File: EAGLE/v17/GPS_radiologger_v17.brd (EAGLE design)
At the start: 40.4 x 26.1 mm, 44 parts, among them IC4 CAT24M01HU5I-GT3, U1 TYPEABZ, U2 BMA400, U4 SPV1050, U5 BME680BME680, U6 CAM-M8Q-0

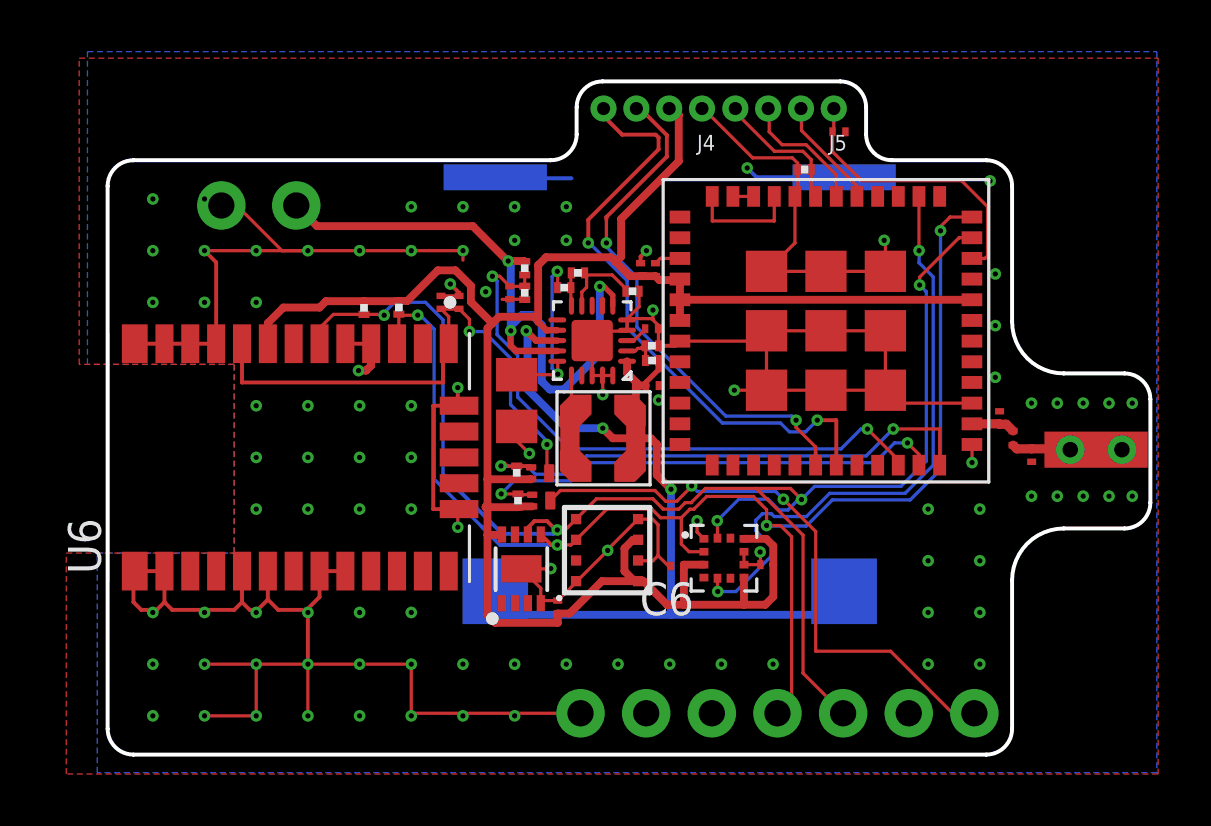
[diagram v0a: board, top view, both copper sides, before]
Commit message: recent board updates
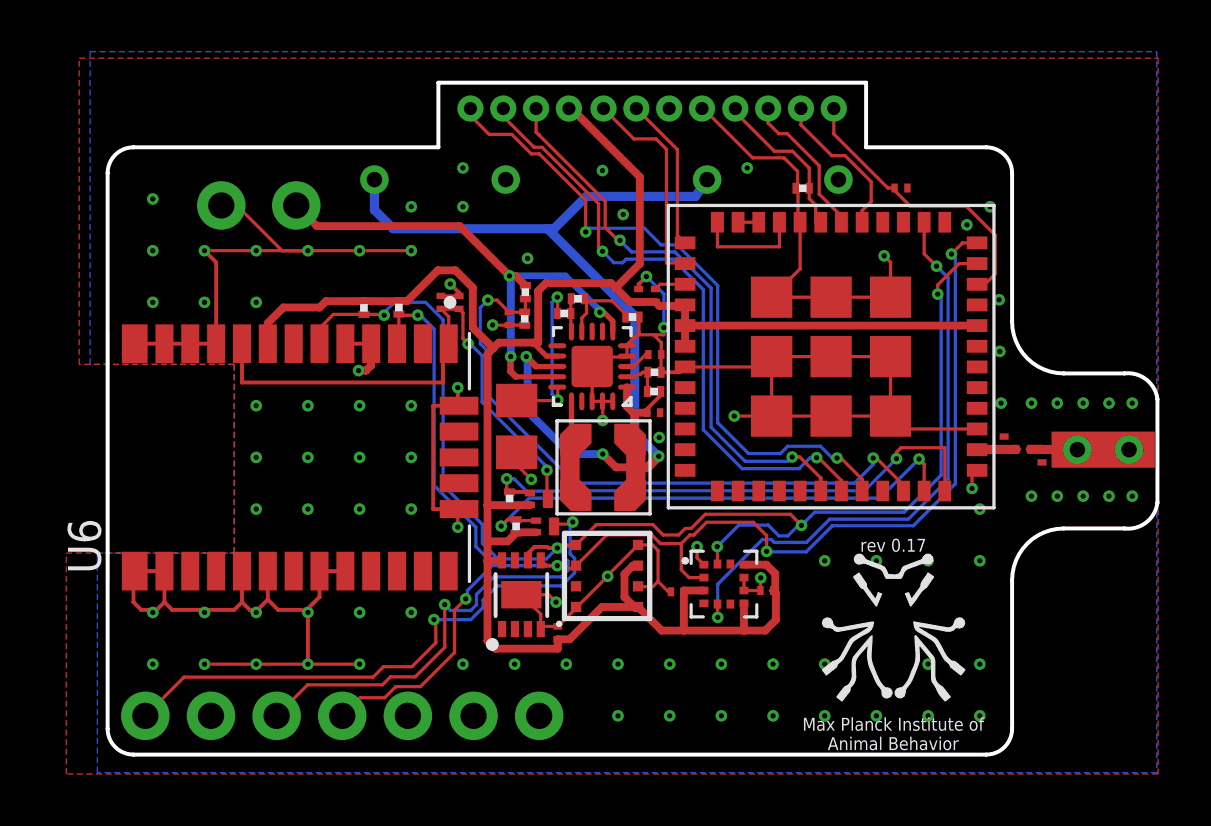
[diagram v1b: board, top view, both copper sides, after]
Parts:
- added J2: (no value), SparkFun-Connectors:1X04_1.27MM_NO_SILK
- U$3, U$4: value ICARUS_V4_RAW -> ICARUS_V4_FOOTPRINT; device TrisolX_Solar_Cells:ICARUS_FULL_TOP -> TrisolX_Solar_Cells:ICARUS_FULL_FOOTPRINT
- moved C1 3.24 mm to (30.7, 21.9)
- moved J7 1.60 mm to (16.7, 1.50), turned to 180 degrees
- moved R8 1.20 mm to (21.1, 14.1)
- moved U$1 1.12 mm to (19.1, 11.1)
- moved C14 1.05 mm to (21.1, 13.2)
- moved R4 1.04 mm to (15.6, 9.91)
- moved R9 1.03 mm to (21.2, 14.8)
- moved U1 1.02 mm to (28.0, 15.4)
- moved PDTA143TMB,1 1.01 mm to (16.9, 8.83)
- moved C4 1.01 mm to (21.2, 15.5)
- moved R5 1.00 mm to (15.8, 8.83)
- moved C9 1.00 mm to (20.5, 17.8)
- moved PDTA143TMB,315 1.00 mm to (16.7, 9.89)
- moved C7 1.00 mm to (15.5, 16.9)
- moved C10 1.00 mm to (21.2, 17.8)
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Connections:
- new net N$18: J4.2
- net DM: now also J4.4
- net DP: now also J4.3
- net GND: now also U$3.P$3, U$4.P$3; no longer U$3.P$2, U$4.P$2
- net POWER: now also J2.1; no longer J4.2
- net RX: now also J2.2; no longer J4.3
- net TX: now also J2.3; no longer J4.4
- net VBUS: now also J2.4
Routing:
- net VBUS: track 0.00 -> 26.0 mm, vias 0 -> 2
- net GND: track 147.3 -> 127.3 mm, vias 97 -> 95
- net DM: track 0.00 -> 8.22 mm
- net SCL: track 60.2 -> 67.1 mm, vias 5 -> 6
- net DP: track 0.00 -> 5.98 mm
- net N$7: track 35.4 -> 40.3 mm
- net BAT: track 25.5 -> 21.0 mm
- net POWER: track 79.8 -> 82.3 mm
- net SDA: track 53.9 -> 56.0 mm, vias 4 -> 5
- net RX: track 20.2 -> 22.0 mm
- net SWDIO: track 4.65 -> 5.97 mm
- net VOLT_MEAS: track 23.5 -> 24.8 mm
- net SCD_PDTA: track 18.8 -> 20.0 mm
- net BOOT: track 5.81 -> 6.67 mm
- net SCD_PWR: track 23.4 -> 22.6 mm
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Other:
- board size 40.4 x 26.1 mm -> 40.6 x 26 mm
- board text added: "Max Planck Institute of Animal Behavior"
- board text added: "rev 0.17"
- board text removed: "Pollution Tag v1.15.0"
